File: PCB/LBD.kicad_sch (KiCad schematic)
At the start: 28 parts, among them J1 USB4155-03-C_REVA, SW1 SW_Push, U1 RP2040, U2 TPSM828214SILR, U3 W25Q128JVSIQ, Y1 Crystal_GND24

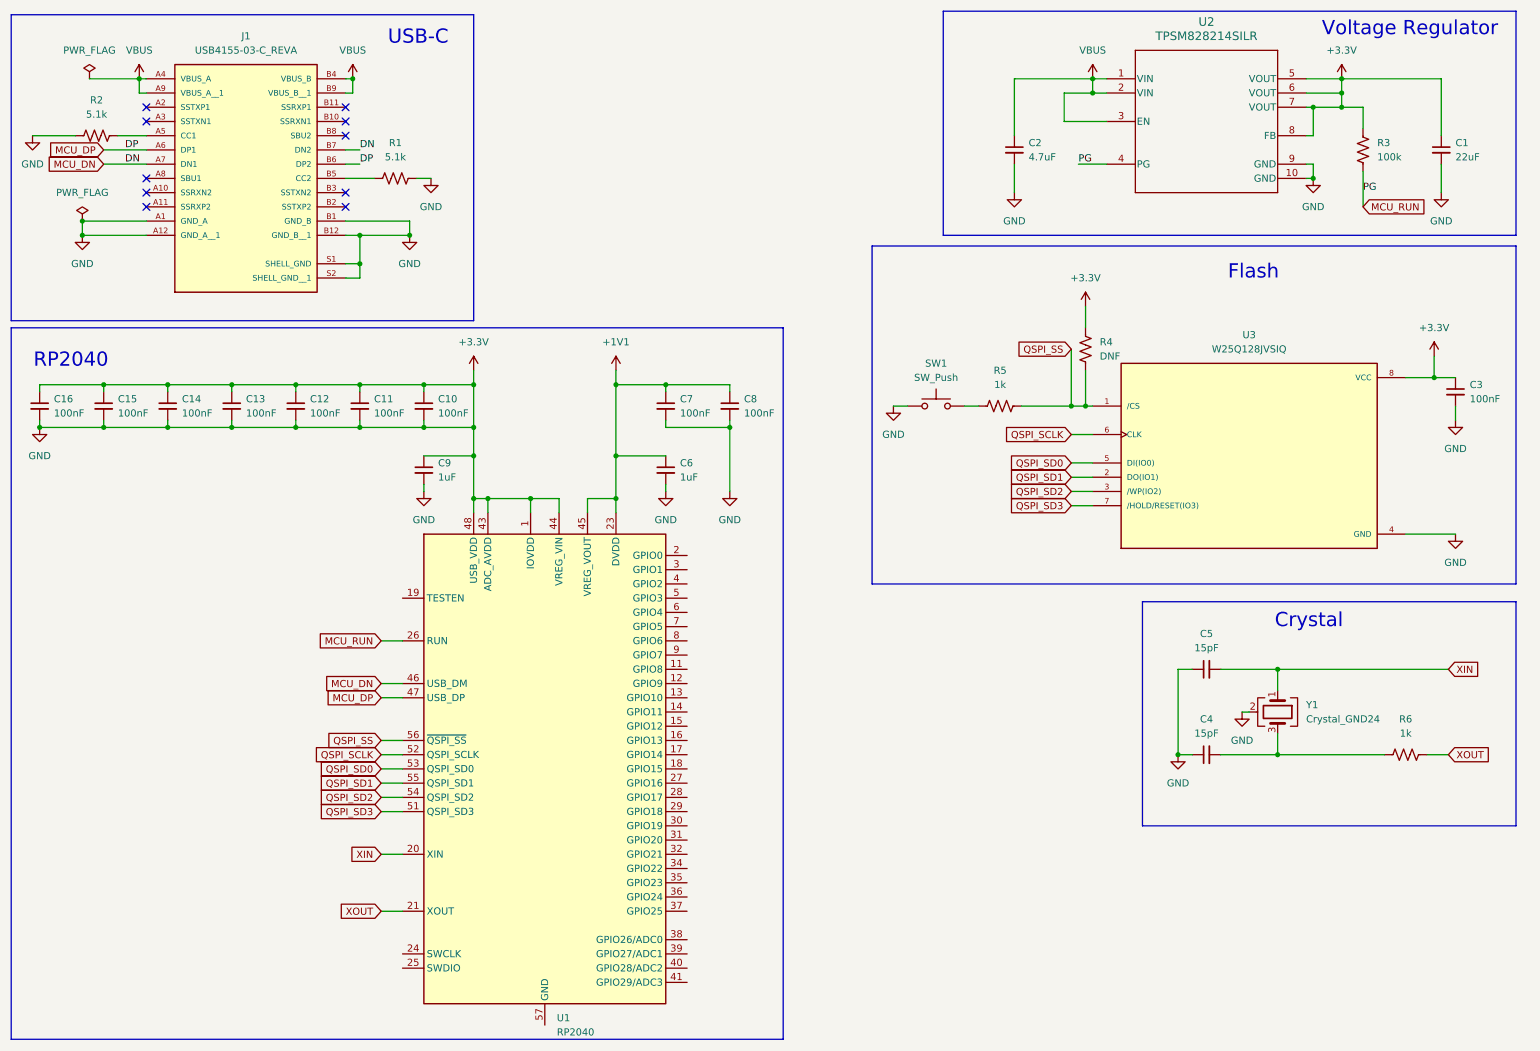
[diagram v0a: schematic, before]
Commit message: i forgot what i changed
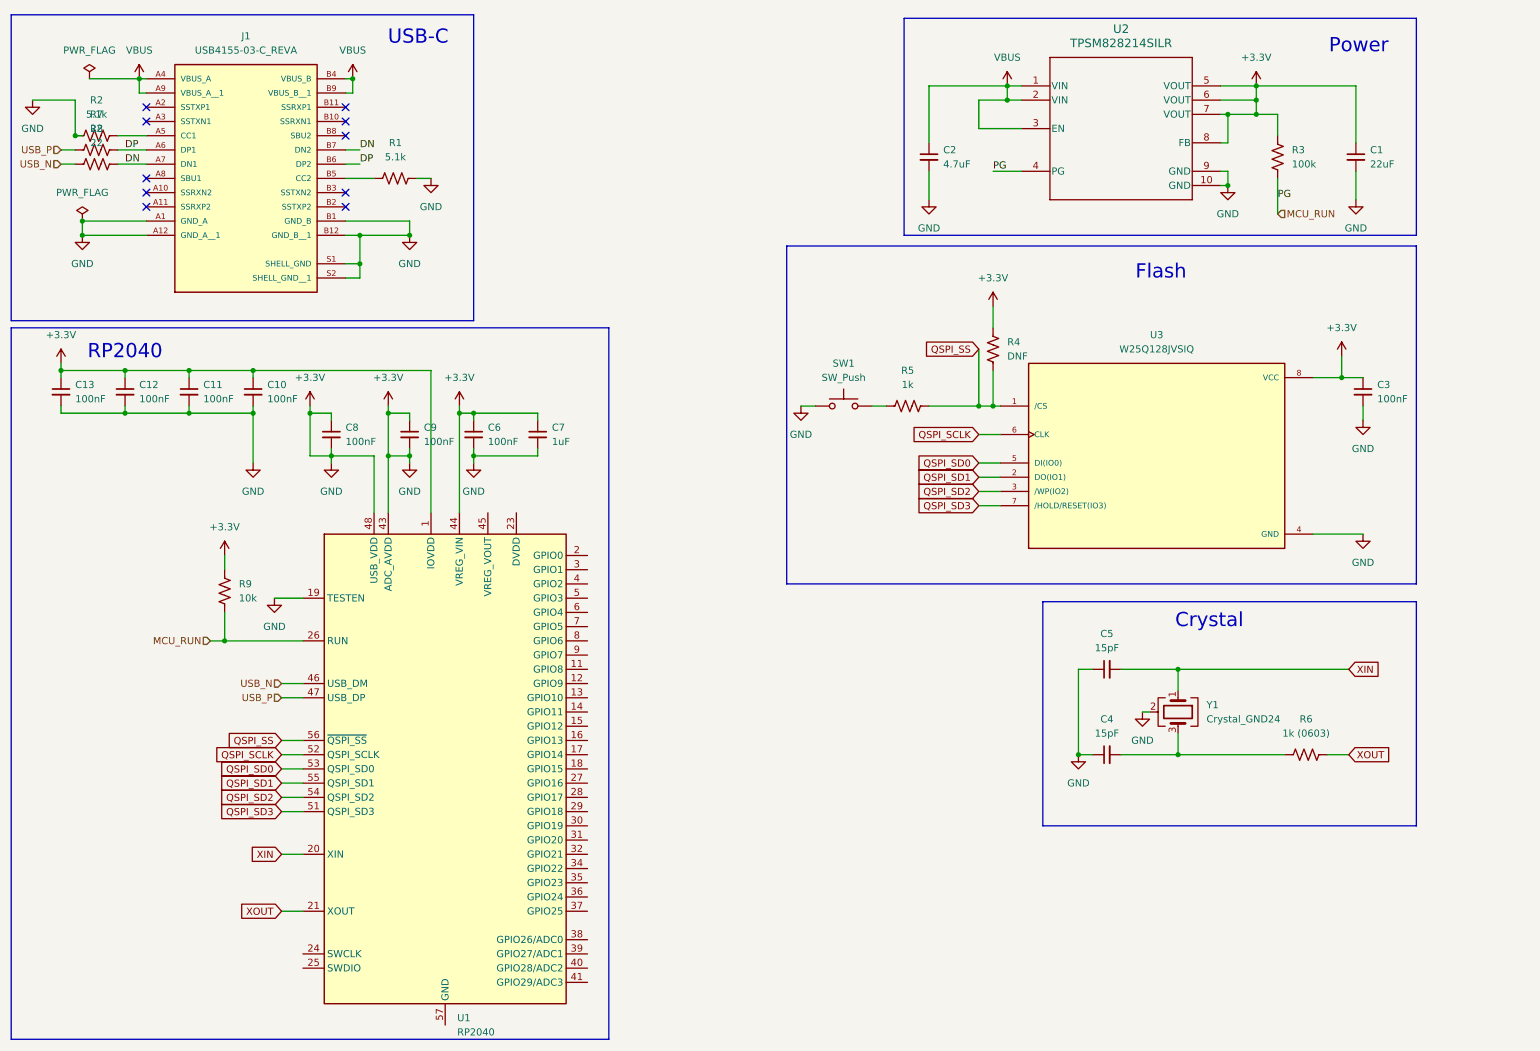
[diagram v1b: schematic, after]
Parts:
- removed C14, C15, C16: 100nF, symbol Device:C_Small
- added R7, R8: 22, symbol Device:R_US
- added R9: 10k, symbol Device:R_US
- C6, C9: value 1uF -> 100nF
- C7: value 100nF -> 1uF
- R6: value 1k -> 1k (0603)
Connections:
- net +3.3V: now also C6.1, C7.1, C8.1, U1.19 (TESTEN), R9.2
- net MCU_RUN: now also R9.1
- removed net +1V1: C6.1, C7.1, C8.1, U1.23 (DVDD), U1.45 (VREG_VOUT), U1.50 (DVDD)
- net MCU_DN renamed DN
- net DN: now also R8.2; no longer U1.46 (USB_DM)
- net MCU_DP renamed DP
- net DP: now also R7.2; no longer U1.47 (USB_DP)
- new net: U1.23 (DVDD), U1.50 (DVDD)
- new net USB_N: R8.1, U1.46 (USB_DM)
- new net USB_P: R7.1, U1.47 (USB_DP)
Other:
- note added: "Power"
- note removed: "Voltage Regulator"
- moved on the sheet: C3, C4, C5, R4, R5, R6, SW1, U1, U3, Y1
